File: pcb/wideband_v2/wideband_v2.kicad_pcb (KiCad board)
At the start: 2 copper layers, 50 x 40 mm, 103 parts, among them J1 DISPLAY, J2 GPIO, J3 LSU, J4 Tag connect, J5 USB, Q1 WSF60N06, SW1 SW_Push, U1 DAC5571IDBVR, U10 XC6206P332MR, U2 L7805, U3 DAC5571IDBVR, U4 RP2040, U5 W25Q128JVS, U6 TXS0102DCU, U7 MCP6004, U8 OPA388IDR, U9 REF3033, Y1 12MHz

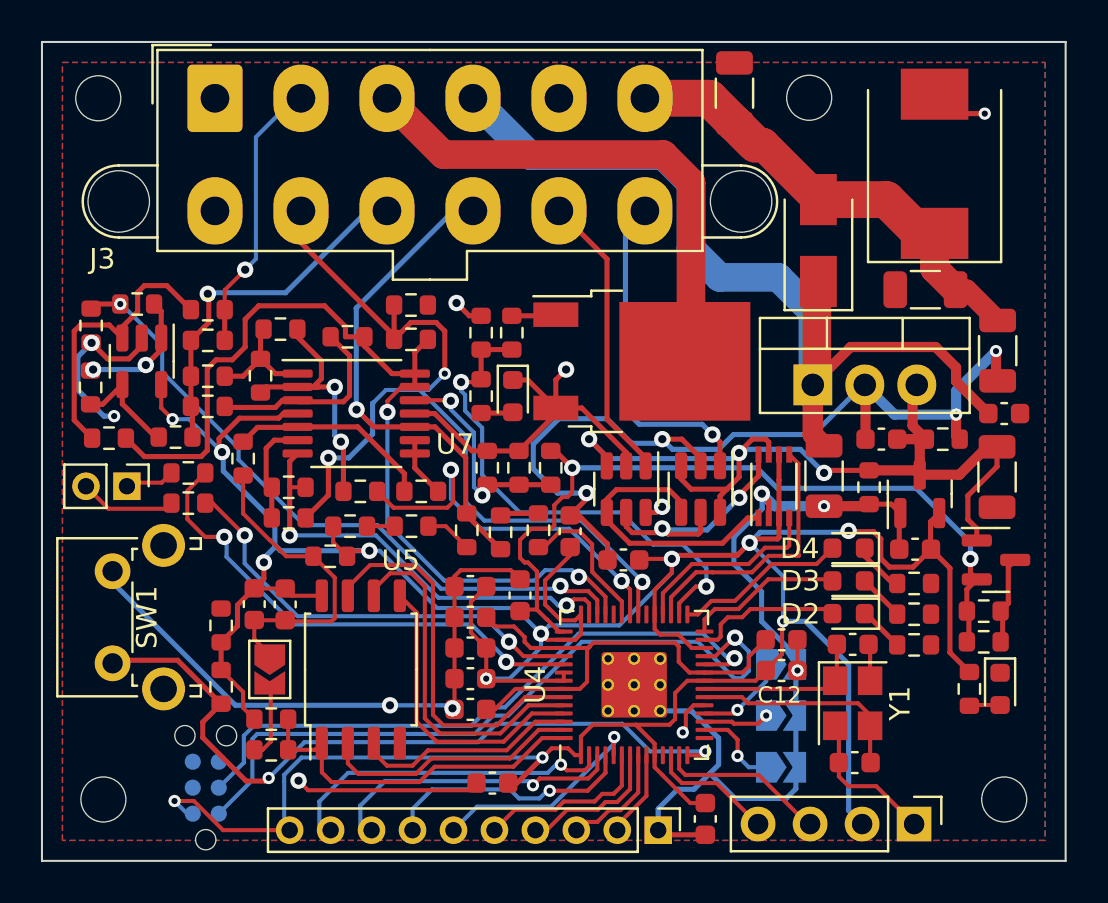
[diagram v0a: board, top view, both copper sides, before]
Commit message: tune tracks/vias
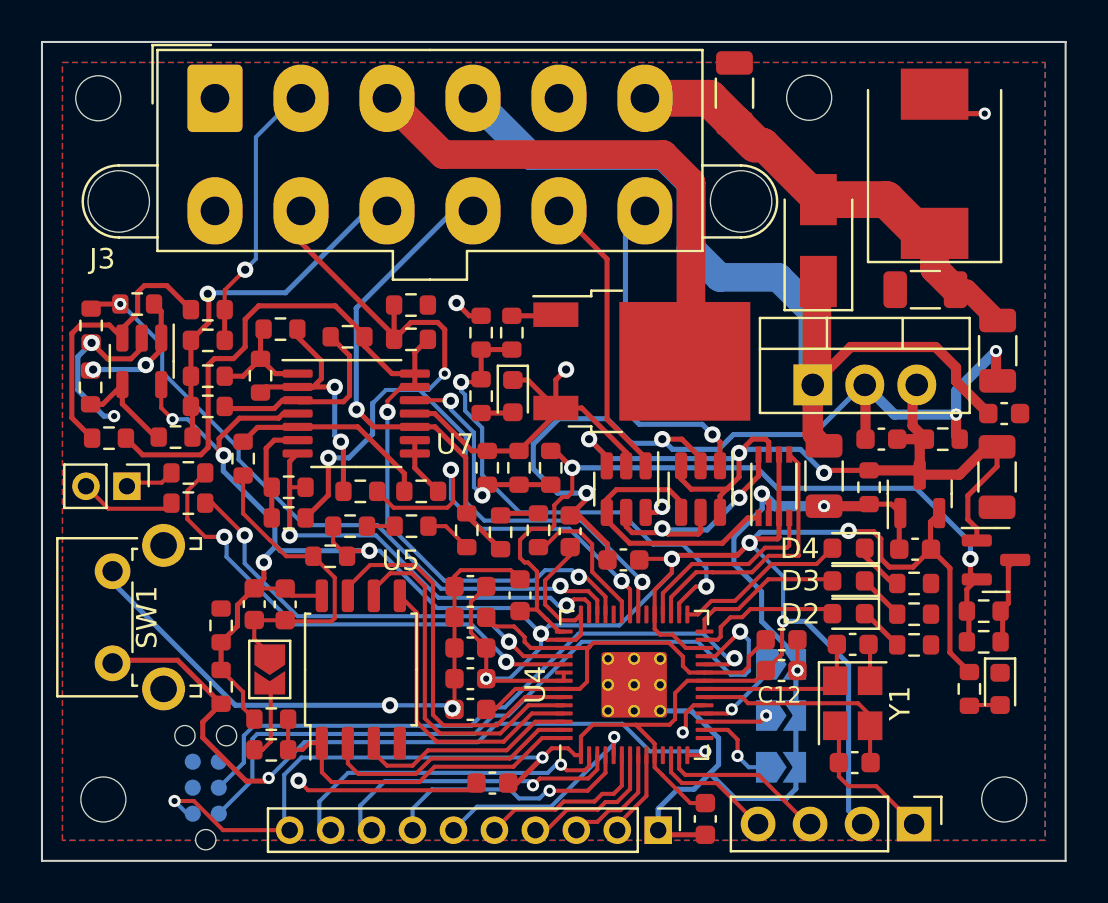
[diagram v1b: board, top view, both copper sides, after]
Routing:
- net Net-(C26-Pad2): track 14.3 -> 13.3 mm
